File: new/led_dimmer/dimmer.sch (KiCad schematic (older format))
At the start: 13 parts

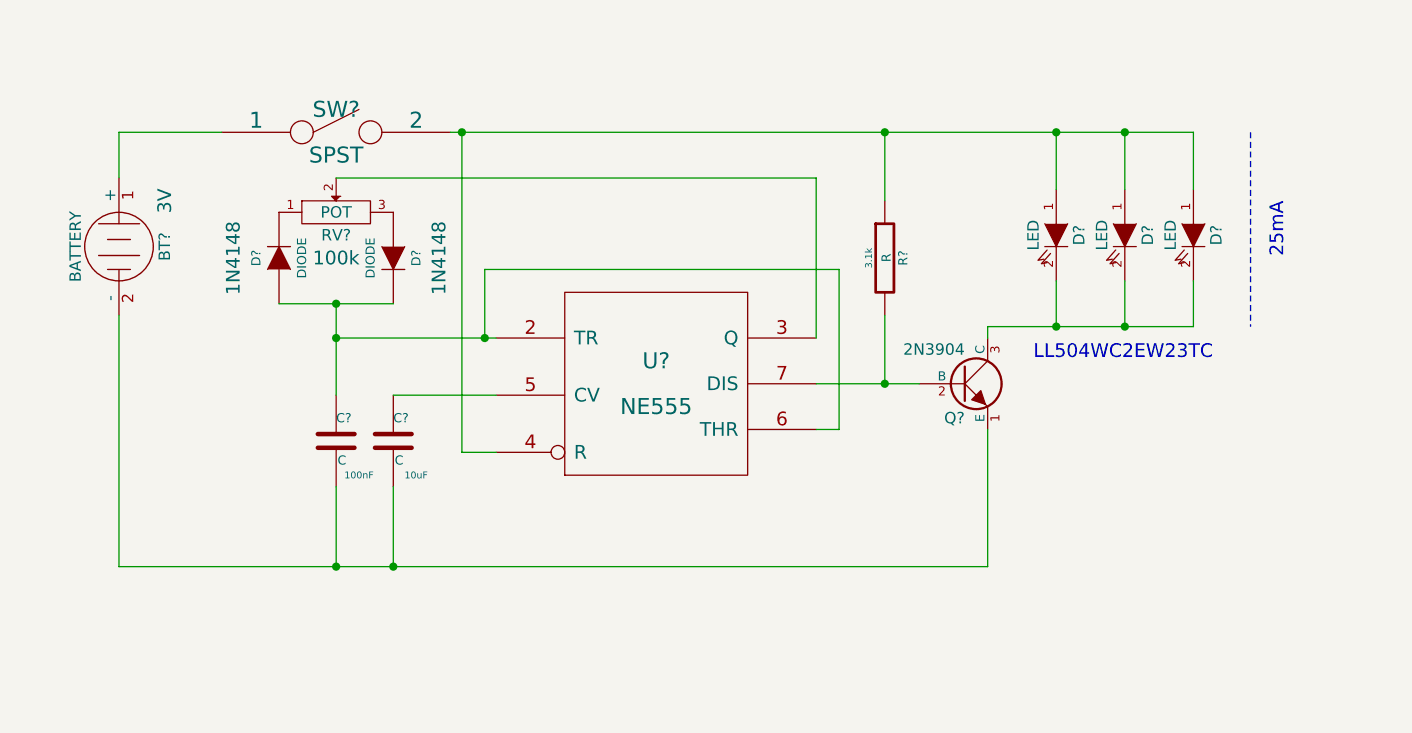
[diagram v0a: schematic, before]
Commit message: .
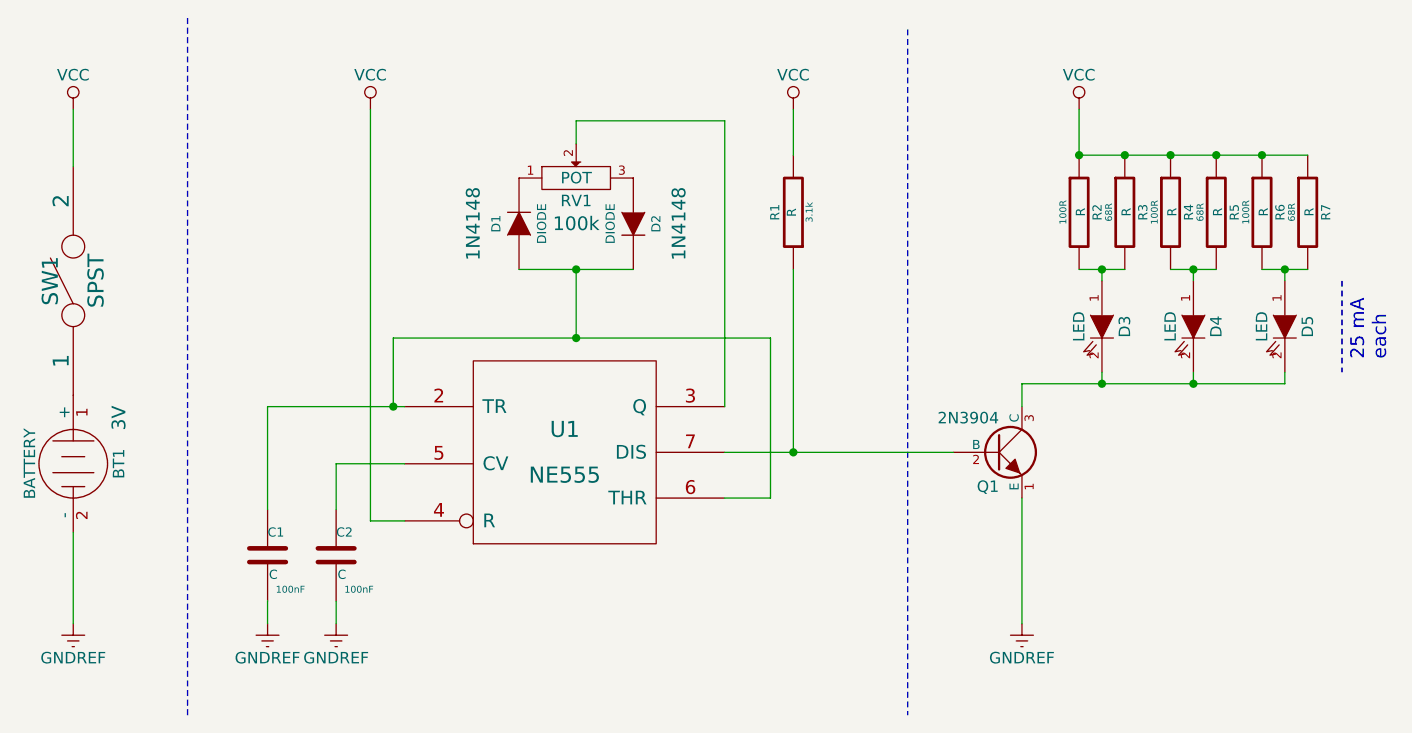
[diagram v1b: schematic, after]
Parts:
- removed BT?: BATTERY, 3V, symbol BATTERY
- removed C?: C, 100nF, symbol C
- removed C?: C, 10uF, symbol C
- removed D? (x2): DIODE, 1N4148, symbol DIODE
- removed D?: LED, ~, symbol LED
- removed D? (x2): LED, symbol LED
- removed Q?: 2N3904, symbol NPN
- removed R?: R, 3.1k, symbol R
- removed RV?: POT, 100k, symbol POT
- removed SW?: SPST, symbol SPST
- removed U?: NE555, symbol LM555N
- added BT1: BATTERY, 3V, symbol BATTERY
- added C1, C2: C, 100nF, symbol C-RESCUE-dimmer
- added D1, D2: DIODE, 1N4148, symbol DIODE
- added D3, D4, D5: LED, symbol LED-RESCUE-dimmer
- added Q1: 2N3904, symbol NPN
- added R1: R, 3.1k, symbol R-RESCUE-dimmer
- added R2, R4, R6: R, 100R, symbol R-RESCUE-dimmer
- added R3, R5, R7: R, 68R, symbol R-RESCUE-dimmer
- added RV1: POT, 100k, symbol POT
- added SW1: SPST, symbol SPST
- added U1: NE555, symbol LM555N
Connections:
- net GND: now also U1.1 (GND)
- net VCC: now also R1.2, R2.1, R3.1, R4.1, R5.1, R6.1, R7.1, SW1.2, U1.4 (R), U1.8 (VCC)
- new net: D3.1 (A), R2.2, R3.2
- new net: D3.2 (K), D4.2 (K), D5.2 (K), Q1.3 (C)
- new net: Q1.2 (B), R1.1, U1.7 (DIS)
- new net: D4.1 (A), R4.2, R5.2
- new net: D5.1 (A), R6.2, R7.2
- new net: C1.1, D1.1 (A), D2.2 (K), U1.2 (TR), U1.6 (THR)
- new net: RV1.2, U1.3 (Q)
- new net: C2.1, U1.5 (CV)
- new net: D1.2 (K), RV1.1
- new net: D2.1 (A), RV1.3
- new net: BT1.1 (+), SW1.1
- new net GNDREF: BT1.2 (-), C1.2, C2.2, Q1.1 (E)
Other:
- note added: "25 mA\neach"
- note removed: "25mA"
- note removed: "LL504WC2EW23TC"
